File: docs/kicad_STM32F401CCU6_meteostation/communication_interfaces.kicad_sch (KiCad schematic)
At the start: 1 part, among them J2 Generic UART Interface

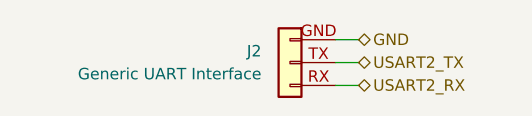
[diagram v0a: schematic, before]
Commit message: docs: Finish M0 Hardware Scheme
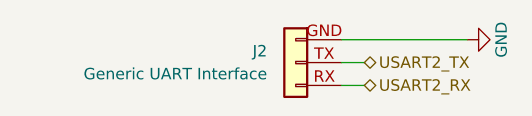
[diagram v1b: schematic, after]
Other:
- title: Communication Interfaces and Protocols Scheme -> Peripheral Interfaces and Protocols Scheme
- moved on the sheet: J2
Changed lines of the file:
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@@
   (paper "A5")
   (title_block
-    (title "Communication Interfaces and Protocols Scheme")
+    (title "Peripheral Interfaces and Protocols Scheme")
+    (date "2026-10-15")
+    (rev "v1.0")
   )
-  (wire (pts (xy 47.625 20.32) (xy 45.085 20.32))
+  (wire (pts (xy 59.69 20.32) (xy 45.72 20.32))
     (stroke (width 0) (type default))
   )
-  (wire (pts (xy 47.625 25.4) (xy 45.085 25.4))
+  (wire (pts (xy 48.26 25.4) (xy 45.72 25.4))
     (stroke (width 0) (type default))
   )
-  (wire (pts (xy 47.625 22.86) (xy 45.085 22.86))
+  (wire (pts (xy 48.26 22.86) (xy 45.72 22.86))
     (stroke (width 0) (type default))
   )
-  (hierarchical_label "GND" (shape bidirectional) (at 47.625 20.32 0) (fields_autoplaced)
+  (hierarchical_label "USART2_RX" (shape bidirectional) (at 48.26 25.4 0) (fields_autoplaced)
     (effects (font (size 1.27 1.27)) (justify left))
   )
-  (hierarchical_label "USART2_RX" (shape bidirectional) (at 47.625 25.4 0) (fields_autoplaced)
+  (hierarchical_label "USART2_TX" (shape bidirectional) (at 48.26 22.86 0) (fields_autoplaced)
     (effects (font (size 1.27 1.27)) (justify left))
   )
-  (hierarchical_label "USART2_TX" (shape bidirectional) (at 47.625 22.86 0) (fields_autoplaced)
-    (effects (font (size 1.27 1.27)) (justify left))
-  )
-  (symbol (lib_id "Connector_Generic:Conn_01x03") (at 40.005 22.86 0) (mirror y) (unit 1)
+  (symbol (lib_id "Connector_Generic:Conn_01x03") (at 40.64 22.86 0) (mirror y) (unit 1)
     (in_bom yes) (on_board yes) (dnp no)
-    (property "Reference" "J2" (at 36.83 21.59 0)
+    (property "Reference" "J2" (at 37.465 21.59 0)
       (effects (font (size 1.27 1.27)) (justify left))
     )
-    (property "Value" "Generic UART Interface" (at 36.83 24.13 0)
+    (property "Value" "Generic UART Interface" (at 37.465 24.13 0)
       (effects (font (size 1.27 1.27)) (justify left))
     )
-    (property "Footprint" "" (at 40.005 22.86 0)
+    (property "Footprint" "" (at 40.64 22.86 0)
       (effects (font (size 1.27 1.27)) hide)
     )
-    (property "Datasheet" "~" (at 40.005 22.86 0)
+    (property "Datasheet" "~" (at 40.64 22.86 0)
       (effects (font (size 1.27 1.27)) hide)
     )
@@
         )
       )
+    )
+  )
+  (symbol (lib_id "power:GND") (at 59.69 20.32 90) (mirror x) (unit 1)
+    (in_bom yes) (on_board yes) (dnp no)
+    (property "Reference" "#PWR01" (at 66.04 20.32 0)
+      (effects (font (size 1.27 1.27)) hide)
+    )
+    (property "Value" "GND" (at 63.5 20.32 0)
+      (effects (font (size 1.27 1.27)))
+    )
+    (property "Footprint" "" (at 59.69 20.32 0)
+      (effects (font (size 1.27 1.27)) hide)
+    )
+    (property "Datasheet" "" (at 59.69 20.32 0)
+      (effects (font (size 1.27 1.27)) hide)
+    )
+    (pin "1")
+    (instances
+      (project "kicad_STM32F401CCU6_meteostation"
+        (path "/d357996e-dbf2-4ea9-a910-dce674dbe94c/e9ee7e41-edae-4378-8334-707fb9ac30d7"
+          (reference "#PWR01") (unit 1)
+        )
+      )
